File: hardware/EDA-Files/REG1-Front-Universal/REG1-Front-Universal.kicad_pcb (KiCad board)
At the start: 2 copper layers, 28.5 x 52.8 mm, 25 parts, among them J1 Frontpanel, SW1 Prog, SW2 Btn1, SW3 Res, SW4 BL

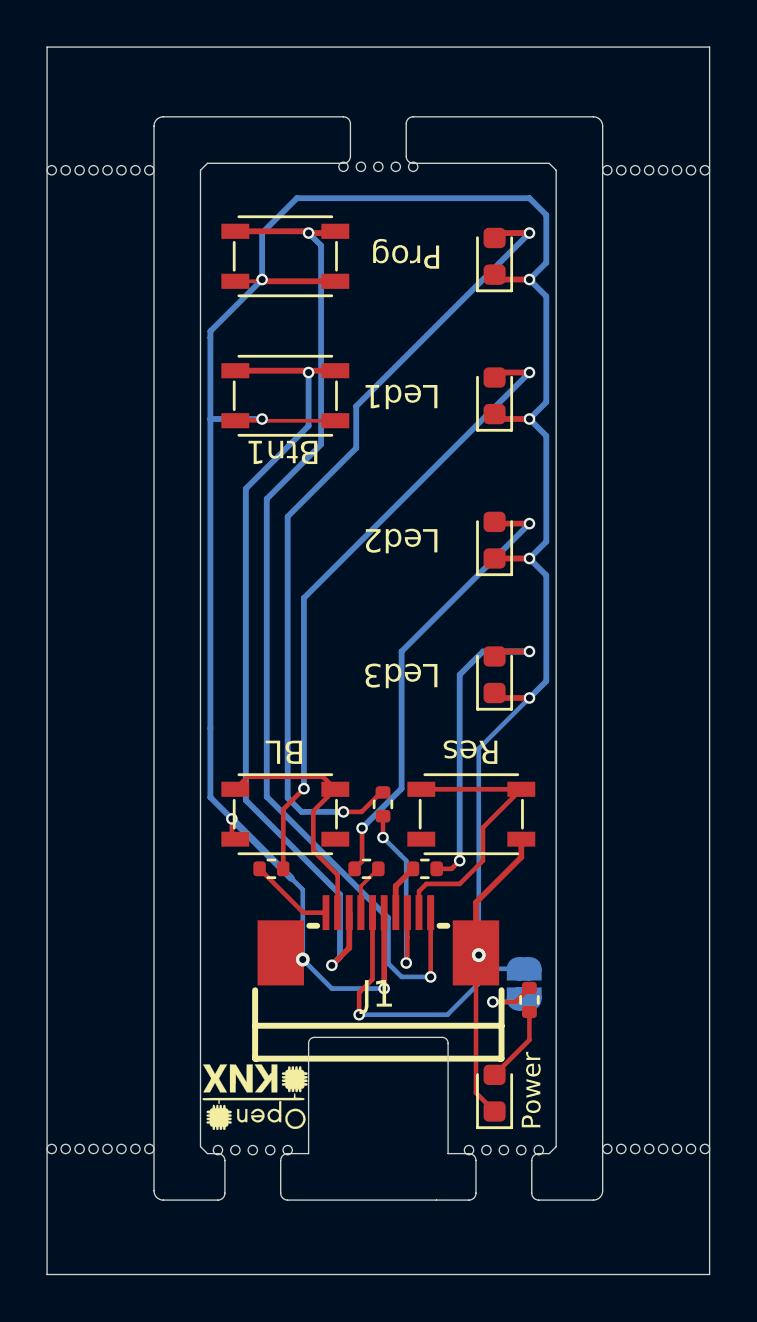
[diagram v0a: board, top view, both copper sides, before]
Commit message: increased size of Front-Universal, WIP
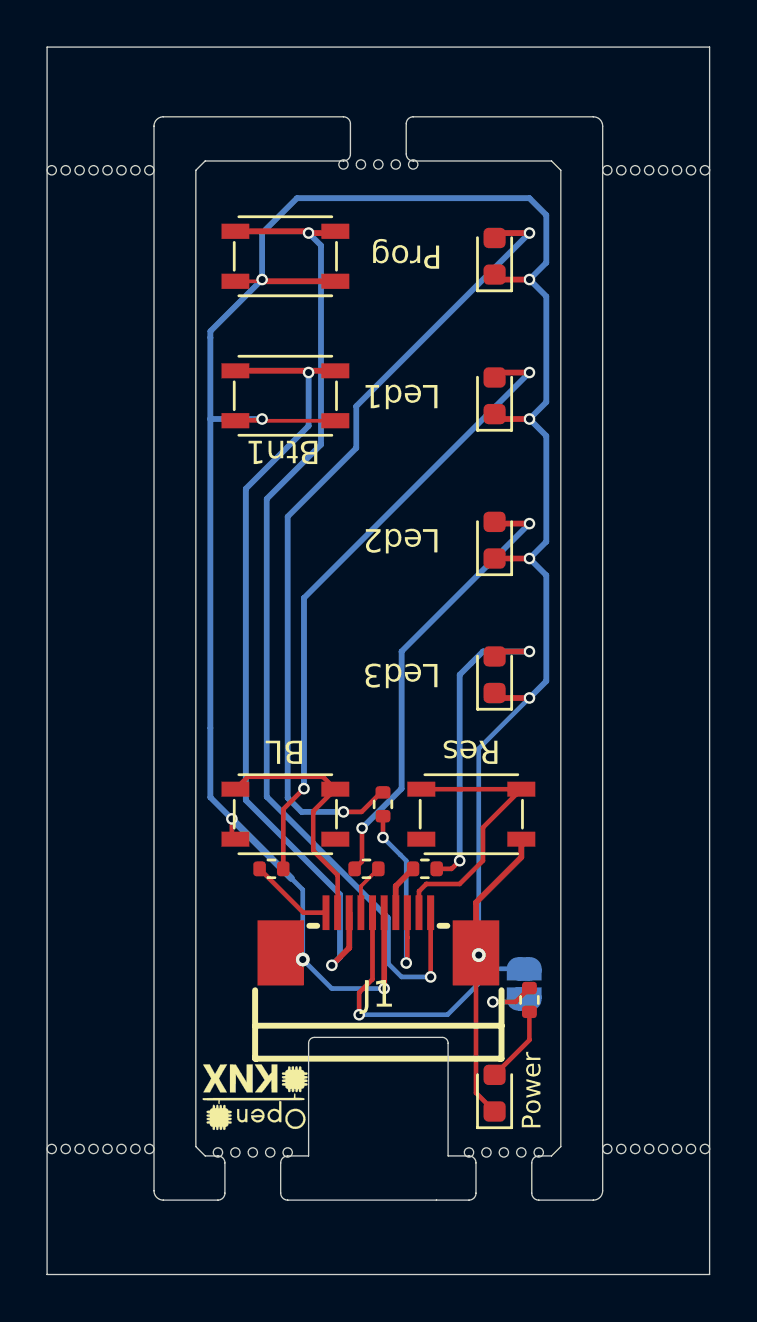
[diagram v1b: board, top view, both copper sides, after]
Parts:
- moved mouse-bite 0.10 mm to (54.0, 42.3)
- moved mouse-bite 0.10 mm to (48.6, 86.3)
- moved mouse-bite 0.10 mm to (59.4, 86.3)
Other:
- outline, holes or cut-outs redrawn
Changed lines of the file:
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@@
   )
   (footprint "DomsKiCADLib:mouse-bite-2.00mm-slot_1side" (layer "F.Cu")
-    (at 48.6 86.2)
+    (at 48.6 86.3)
     (attr through_hole board_only exclude_from_pos_files exclude_from_bom)
     (fp_text reference "mouse-bite" (at 0.2 2.5) (layer "F.SilkS") hide
@@
   )
   (footprint "DomsKiCADLib:mouse-bite-2.00mm-slot_1side" (layer "F.Cu")
-    (at 59.4 86.2)
+    (at 59.4 86.3)
     (attr through_hole board_only exclude_from_pos_files exclude_from_bom)
     (fp_text reference "mouse-bite" (at 0.4 2.8) (layer "F.SilkS") hide
@@
   )
   (footprint "DomsKiCADLib:mouse-bite-2.00mm-slot_1side" (layer "F.Cu")
-    (at 54 42.4 180)
+    (at 54 42.3 180)
     (attr through_hole board_only exclude_from_pos_files exclude_from_bom)
     (fp_text reference "mouse-bite" (at 0.2 2.2) (layer "F.SilkS") hide
@@
   (gr_line (start 45 71) (end 73.25 71)
     (stroke (width 0.1) (type default)) (layer "Eco1.User"))
-  (gr_line (start 46.35 85.3) (end 46.35 43.3)
+  (gr_line (start 46.15 85.3) (end 46.15 43.3)
     (stroke (width 0.05) (type solid)) (layer "Edge.Cuts"))
   (gr_line (start 63.25 41) (end 55.5 41)
@@
   (gr_line (start 56.5 87.6) (end 57.9 87.6)
     (stroke (width 0.05) (type solid)) (layer "Edge.Cuts"))
-  (gr_line (start 61.35 85.6) (end 60.9 85.6)
+  (gr_line (start 61.45 85.7) (end 60.9 85.7)
     (stroke (width 0.05) (type solid)) (layer "Edge.Cuts"))
-  (gr_line (start 51 85.6) (end 50.1 85.6)
+  (gr_line (start 51 85.7) (end 50.1 85.7)
     (stroke (width 0.05) (type solid)) (layer "Edge.Cuts"))
   (gr_line (start 50.1 87.6) (end 56.5 87.6)
     (stroke (width 0.05) (type solid)) (layer "Edge.Cuts"))
-  (gr_arc (start 52.8 42.7) (mid 52.712132 42.912132) (end 52.5 43)
+  (gr_arc (start 52.8 42.6) (mid 52.712132 42.812132) (end 52.5 42.9)
     (stroke (width 0.05) (type default)) (layer "Edge.Cuts"))
-  (gr_line (start 61.35 43) (end 55.5 43)
+  (gr_line (start 61.45 42.9) (end 55.5 42.9)
     (stroke (width 0.05) (type default)) (layer "Edge.Cuts"))
-  (gr_line (start 46.65 43) (end 46.35 43.3)
+  (gr_line (start 46.55 42.9) (end 46.15 43.3)
     (stroke (width 0.05) (type solid)) (layer "Edge.Cuts"))
-  (gr_arc (start 47.1 85.6) (mid 47.312132 85.687868) (end 47.4 85.9)
+  (gr_arc (start 47.1 85.7) (mid 47.312132 85.787868) (end 47.4 86)
     (stroke (width 0.05) (type default)) (layer "Edge.Cuts"))
-  (gr_line (start 61.65 85.3) (end 61.35 85.6)
+  (gr_line (start 61.85 85.3) (end 61.45 85.7)
     (stroke (width 0.05) (type solid)) (layer "Edge.Cuts"))
   (gr_arc (start 52.5 41) (mid 52.712132 41.087868) (end 52.8 41.3)
@@
   (gr_arc (start 63.25 41) (mid 63.532843 41.117157) (end 63.65 41.4)
     (stroke (width 0.05) (type default)) (layer "Edge.Cuts"))
-  (gr_line (start 46.65 85.6) (end 46.35 85.3)
+  (gr_line (start 46.55 85.7) (end 46.15 85.3)
     (stroke (width 0.05) (type default)) (layer "Edge.Cuts"))
   (gr_line (start 51.25 80.6) (end 56.75 80.6)
@@
   (gr_arc (start 60.9 87.6) (mid 60.687868 87.512132) (end 60.6 87.3)
     (stroke (width 0.05) (type default)) (layer "Edge.Cuts"))
-  (gr_arc (start 49.8 85.9) (mid 49.887868 85.687868) (end 50.1 85.6)
+  (gr_arc (start 49.8 86) (mid 49.887868 85.787868) (end 50.1 85.7)
     (stroke (width 0.05) (type default)) (layer "Edge.Cuts"))
   (gr_arc (start 63.65 87.2) (mid 63.532843 87.482843) (end 63.25 87.6)
     (stroke (width 0.05) (type default)) (layer "Edge.Cuts"))
-  (gr_arc (start 55.5 43) (mid 55.287868 42.912132) (end 55.2 42.7)
+  (gr_arc (start 55.5 42.9) (mid 55.287868 42.812132) (end 55.2 42.6)
     (stroke (width 0.05) (type default)) (layer "Edge.Cuts"))
-  (gr_line (start 61.65 43.3) (end 61.65 85.3)
+  (gr_line (start 61.85 43.3) (end 61.85 85.3)
     (stroke (width 0.05) (type solid)) (layer "Edge.Cuts"))
-  (gr_line (start 51 85.6) (end 51 80.85)
+  (gr_line (start 51 85.7) (end 51 80.85)
     (stroke (width 0.05) (type default)) (layer "Edge.Cuts"))
-  (gr_line (start 60.6 85.9) (end 60.6 87.3)
+  (gr_line (start 60.6 86) (end 60.6 87.3)
     (stroke (width 0.05) (type default)) (layer "Edge.Cuts"))
-  (gr_line (start 57.9 85.6) (end 57 85.6)
+  (gr_line (start 57.9 85.7) (end 57 85.7)
     (stroke (width 0.05) (type default)) (layer "Edge.Cuts"))
-  (gr_line (start 58.2 87.3) (end 58.2 85.9)
+  (gr_line (start 58.2 87.3) (end 58.2 86)
     (stroke (width 0.05) (type default)) (layer "Edge.Cuts"))
   (gr_arc (start 58.2 87.3) (mid 58.112132 87.512132) (end 57.9 87.6)
@@
   (gr_line (start 52.5 41) (end 44.75 41)
     (stroke (width 0.05) (type solid)) (layer "Edge.Cuts"))
-  (gr_line (start 46.65 43) (end 52.5 43)
+  (gr_line (start 46.55 42.9) (end 52.5 42.9)
     (stroke (width 0.05) (type solid)) (layer "Edge.Cuts"))
-  (gr_line (start 57 80.85) (end 57 85.6)
+  (gr_line (start 57 80.85) (end 57 85.7)
     (stroke (width 0.05) (type default)) (layer "Edge.Cuts"))
-  (gr_line (start 52.8 42.7) (end 52.8 41.3)
+  (gr_line (start 52.8 42.6) (end 52.8 41.3)
     (stroke (width 0.05) (type default)) (layer "Edge.Cuts"))
-  (gr_arc (start 60.6 85.9) (mid 60.687868 85.687868) (end 60.9 85.6)
+  (gr_arc (start 60.6 86) (mid 60.687868 85.787868) (end 60.9 85.7)
     (stroke (width 0.05) (type default)) (layer "Edge.Cuts"))
-  (gr_line (start 47.4 87.3) (end 47.4 85.9)
+  (gr_line (start 47.4 87.3) (end 47.4 86)
     (stroke (width 0.05) (type default)) (layer "Edge.Cuts"))
-  (gr_line (start 49.8 85.9) (end 49.8 87.3)
+  (gr_line (start 49.8 86) (end 49.8 87.3)
     (stroke (width 0.05) (type default)) (layer "Edge.Cuts"))
-  (gr_line (start 47.1 85.6) (end 46.65 85.6)
+  (gr_line (start 47.1 85.7) (end 46.55 85.7)
     (stroke (width 0.05) (type solid)) (layer "Edge.Cuts"))
   (gr_line (start 60.9 87.6) (end 63.25 87.6)
@@
   (gr_line (start 63.65 87.2) (end 63.65 41.4)
     (stroke (width 0.05) (type solid)) (layer "Edge.Cuts"))
-  (gr_line (start 61.35 43) (end 61.65 43.3)
+  (gr_line (start 61.45 42.9) (end 61.85 43.3)
     (stroke (width 0.05) (type default)) (layer "Edge.Cuts"))
-  (gr_arc (start 57.9 85.6) (mid 58.112132 85.687868) (end 58.2 85.9)
+  (gr_arc (start 57.9 85.7) (mid 58.112132 85.787868) (end 58.2 86)
     (stroke (width 0.05) (type default)) (layer "Edge.Cuts"))
   (gr_line (start 44.35 87.2) (end 44.35 41.4)
     (stroke (width 0.05) (type solid)) (layer "Edge.Cuts"))
-  (gr_line (start 55.2 41.3) (end 55.2 42.7)
+  (gr_line (start 55.2 41.3) (end 55.2 42.6)
     (stroke (width 0.05) (type default)) (layer "Edge.Cuts"))
   (gr_arc (start 44.75 87.6) (mid 44.467157 87.482843) (end 44.35 87.2)
